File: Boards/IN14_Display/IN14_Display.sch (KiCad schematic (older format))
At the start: 46 parts, among them IC1 TPIC6B596DW, IC2 TPIC6B596DW, IC3 TPIC6B596DW, IC4 TPIC6B596DW, IC5 TPIC6B596DW, IC6 TPIC6B596DW, IC7 TPIC6B596DW, IC8 TPIC6B596DW, P1 CONN_01X02, P2 CONN_01X06, Q1 BC817

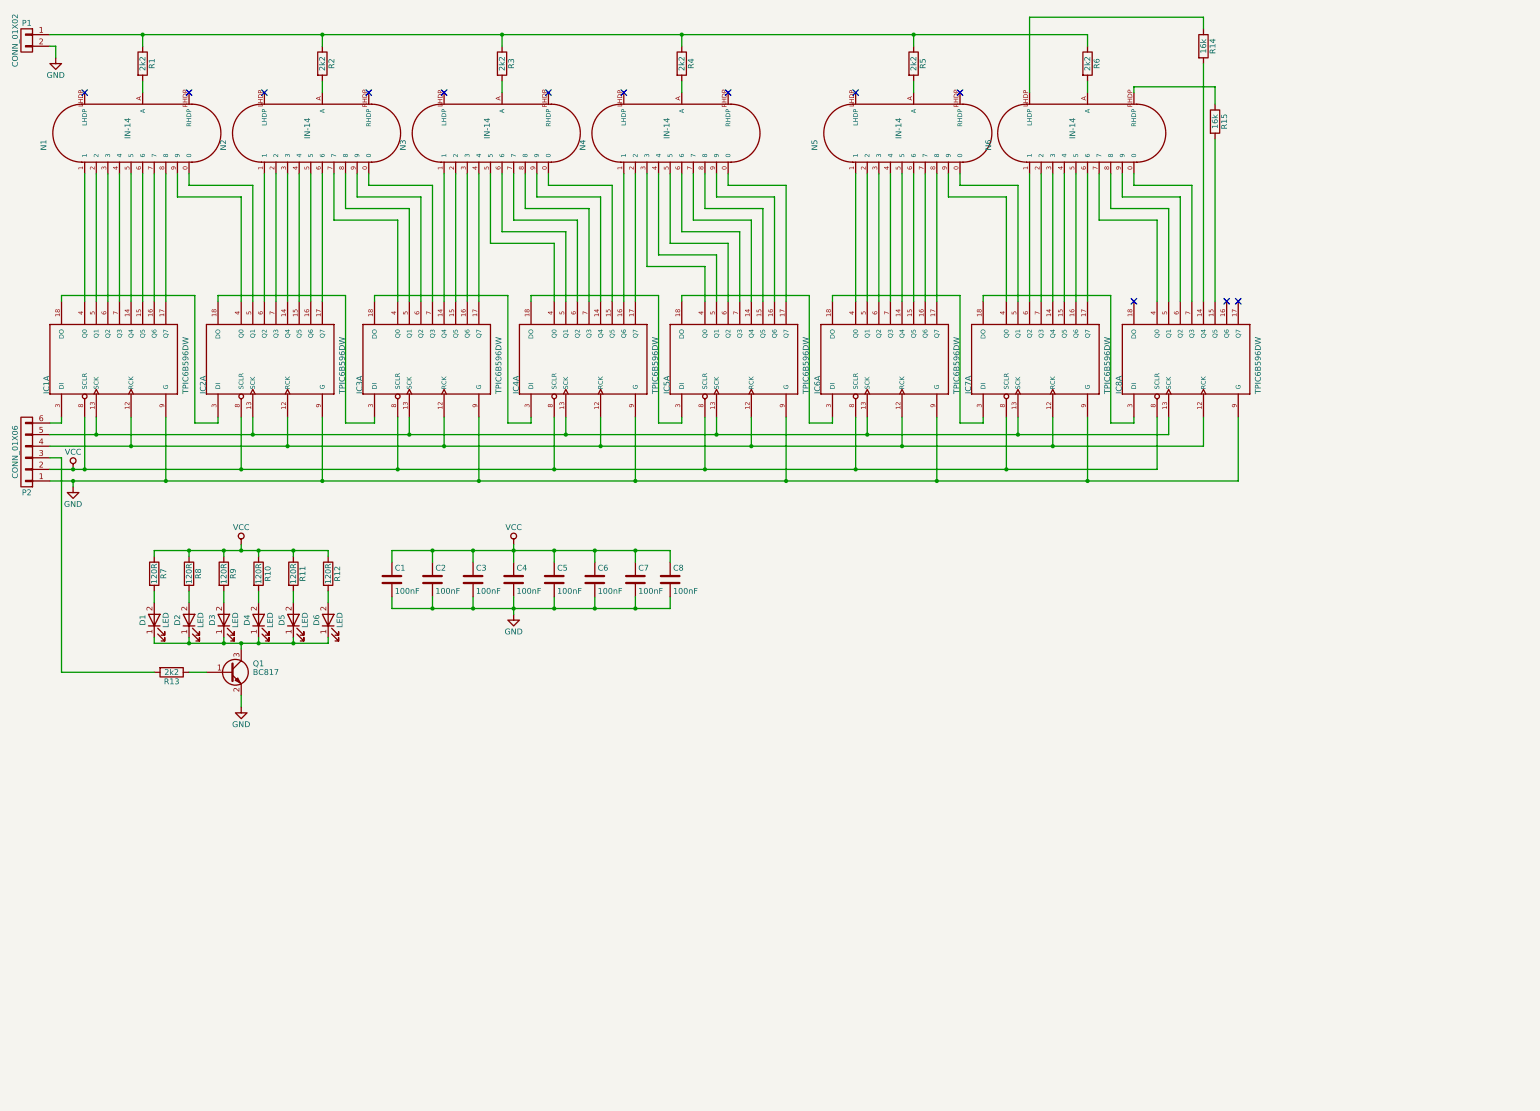
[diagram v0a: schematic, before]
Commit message: Layout done, before PCB order
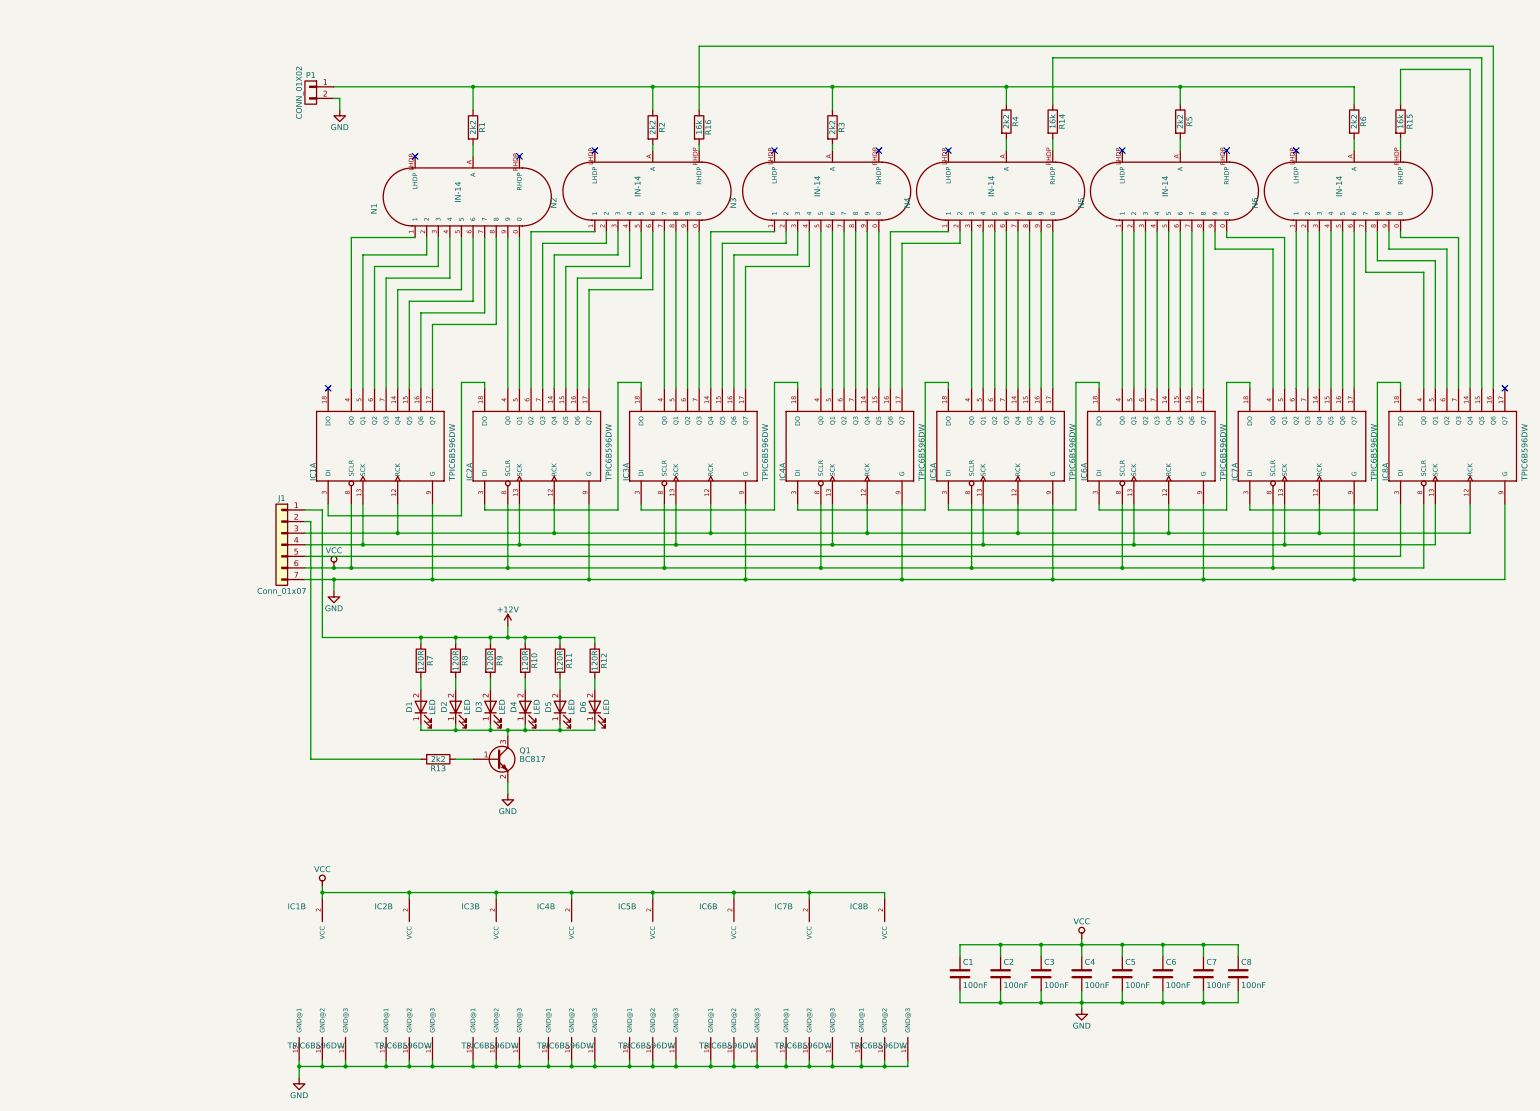
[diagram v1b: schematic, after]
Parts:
- removed P2: CONN_01X06, Pin_Headers:Pin_Header_Straight_1x06_Pitch2.54mm, symbol CONN_01X06
- added unit 2 of IC1
- added unit 2 of IC2
- added unit 2 of IC3
- added unit 2 of IC4
- added unit 2 of IC5
- added unit 2 of IC6
- added unit 2 of IC7
- added unit 2 of IC8
- added J1: Conn_01x07, Pin_Headers:Pin_Header_Straight_1x07_Pitch2.54mm, symbol Conn_01x07
- added R16: 16k, Resistors_SMD:R_0805, symbol R
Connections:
- net GND: now also IC1.10 (GND@2), IC1.11 (GND@3), IC1.19 (GND@1), IC2.10 (GND@2), IC2.11 (GND@3), IC2.19 (GND@1), IC3.10 (GND@2), IC3.11 (GND@3), IC3.19 (GND@1), IC4.10 (GND@2), IC4.11 (GND@3), IC4.19 (GND@1), IC5.10 (GND@2), IC5.11 (GND@3), IC5.19 (GND@1), IC6.10 (GND@2), IC6.11 (GND@3), IC6.19 (GND@1), IC7.10 (GND@2), IC7.11 (GND@3), IC7.19 (GND@1), IC8.10 (GND@2), IC8.11 (GND@3), IC8.19 (GND@1), J1.7 (Pin_7)
- net VCC: now also IC1.2 (VCC), IC2.2 (VCC), IC3.2 (VCC), IC4.2 (VCC), IC5.2 (VCC), IC6.2 (VCC), IC7.2 (VCC), IC8.2 (VCC), J1.6 (Pin_6); no longer R10.1, R11.1, R12.1, R7.1, R8.1, R9.1
- net at N2.RHDP: now also R16.2
- net at N4.RHDP: now also R14.2
- net at N6.LHDP: no longer R14.1
- net at N6.RHDP: now also R15.2; no longer R15.1
- net at R13.2: now also J1.2 (Pin_2)
- net at IC1.12 (RCK), IC2.12 (RCK), IC3.12 (RCK)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: now also J1.3 (Pin_3)
- net at IC1.13 (SCK), IC2.13 (SCK), IC3.13 (SCK)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: now also J1.4 (Pin_4)
- net at IC1.3 (DI): now also IC2.18 (DO)
- net at IC1.18 (DO): no longer IC2.3 (DI)
- net at IC3.3 (DI): now also IC4.18 (DO); no longer IC2.18 (DO)
- net at IC3.18 (DO): now also IC2.3 (DI); no longer IC4.3 (DI)
- net at IC5.3 (DI): now also IC6.18 (DO); no longer IC4.18 (DO)
- net at IC5.18 (DO): now also IC4.3 (DI); no longer IC6.3 (DI)
- net at IC7.3 (DI): now also IC8.18 (DO); no longer IC6.18 (DO)
- net at IC7.18 (DO): now also IC6.3 (DI); no longer IC8.3 (DI)
- net at IC8.14 (Q4): now also R15.1; no longer R14.2
- net at IC8.15 (Q5): now also R14.1; no longer R15.2
- net at IC8.16 (Q6): now also R16.1
- new net: IC8.3 (DI), J1.5 (Pin_5)
- new net +12V: J1.1 (Pin_1), R10.1, R11.1, R12.1, R7.1, R8.1, R9.1
- no-connect marks 13 -> 11
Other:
- moved on the sheet: C1, C2, C3, C4, C5, C6, C7, C8, D1, D2, D3, D4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
